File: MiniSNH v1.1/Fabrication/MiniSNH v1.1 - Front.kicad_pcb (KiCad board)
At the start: 2 copper layers, 20 x 128.5 mm, 11 parts

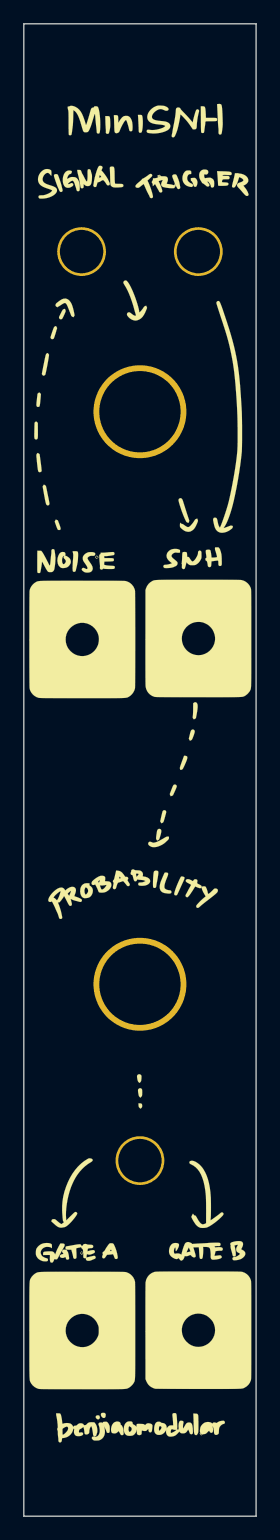
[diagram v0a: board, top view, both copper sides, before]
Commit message: Added gerber files for v1.1
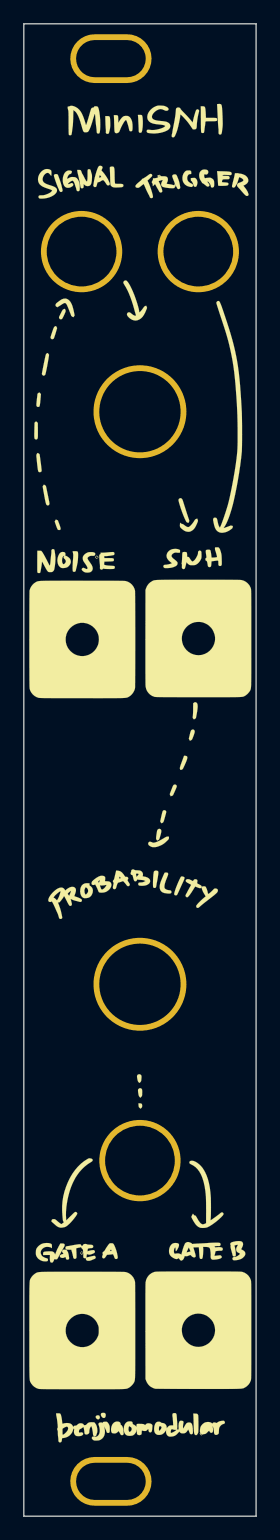
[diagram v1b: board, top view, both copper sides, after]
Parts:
- added REF**: Panel_4HP, benjiaomodular:Panel_4HP, F.Cu at (110.0, 49.0)
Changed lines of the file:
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@@
   )
   (paper "A4")
+  (title_block
+    (title "MiniSNH")
+    (date "2023-06-07")
+    (rev "V1.1")
+    (company "benjiaomodular")
+  )
   (layers
     (0 "F.Cu" signal)
@@
     )
     (pad_to_mask_clearance 0)
-    (grid_origin 110 49)
     (pcbplotparams
       (layerselection 0x00010fc_ffffffff)
@@
       (drillshape 0)
       (scaleselection 1)
-      (outputdirectory "")
+      (outputdirectory "./MiniSNH v1.1 - Front")
     )
   )
@@
       (effects (font (size 1.27 1.27) (thickness 0.15)))
     )
-    (pad "1" thru_hole circle locked (at 0 0) (size 4.2 4.2) (drill 3.735001) (layers *.Cu *.Mask))
+    (pad "1" thru_hole circle locked (at 0 0) (size 7 7) (drill 6) (layers *.Cu *.Mask))
   )
   (footprint "Wire_Pads:SolderWirePad_single_0-8mmDrill" (layer "F.Cu")
@@
       (effects (font (size 1.27 1.27) (thickness 0.15)))
     )
-    (pad "5" thru_hole circle locked (at 0 0) (size 4.2 4.2) (drill 3.735001) (layers *.Cu *.Mask))
+    (pad "5" thru_hole circle locked (at 0 0) (size 7 7) (drill 6) (layers *.Cu *.Mask))
   )
   (footprint "LOGO" (layer "F.Cu")
@@
       (effects (font (size 1.27 1.27) (thickness 0.15)))
     )
-    (pad "3" thru_hole circle locked (at 0 0) (size 4.2 4.2) (drill 3.735001) (layers *.Cu *.Mask))
+    (pad "3" thru_hole circle locked (at 0 0) (size 7 7) (drill 6) (layers *.Cu *.Mask))
   )
   (footprint "LOGO" (layer "F.Cu")
@@
       ) (layer "F.Mask") (width 0.01) (fill solid))
   )
+  (footprint "benjiaomodular:Panel_4HP" (layer "F.Cu")
+    (at 110 49)
+    (attr through_hole)
+    (fp_text reference "REF**" (at 18 -1) (layer "F.Fab") hide
+      (effects (font (size 1 1) (thickness 0.15)))
+    )
+    (fp_text value "Panel_4HP" (at 4 -1) (layer "F.Fab")
+      (effects (font (size 1 1) (thickness 0.15)))
+    )
+    (fp_text user "Clearance for 2020 Aluminum Extrusion" (at 10.5 11.5) (layer "Dwgs.User")
+      (effects (font (size 0.8 0.8) (thickness 0.12)))
+    )
+    (fp_text user "Clearance for 2020 Aluminum Extrusion" (at 10.5 116.5) (layer "Dwgs.User")
+      (effects (font (size 0.8 0.8) (thickness 0.12)))
+    )
+    (fp_line (start 0 128.5) (end 0 0) (layer "Dwgs.User") (width 0.12))
+    (fp_line (start 20 0) (end 20 128.5) (layer "Dwgs.User") (width 0.12))
+    (fp_line (start 0 125.5) (end 20 125.5) (layer "Dwgs.User") (width 0.12))
+    (fp_line (start 0 13) (end 20 13) (layer "Dwgs.User") (width 0.12))
+    (fp_line (start 0 3) (end 20 3) (layer "Dwgs.User") (width 0.12))
+    (fp_line (start 0 115.5) (end 20 115.5) (layer "Dwgs.User") (width 0.12))
+    (fp_line (start 0 0) (end 20 0) (layer "Dwgs.User") (width 0.12))
+    (fp_line (start 20 128.5) (end 0 128.5) (layer "Dwgs.User") (width 0.12))
+    (pad "" thru_hole oval locked (at 7.5 125.5) (size 7 4.2) (drill oval 6 3.2) (layers *.Cu *.Mask))
+    (pad "" thru_hole oval locked (at 7.5 3) (size 7 4.2) (drill oval 6 3.2) (layers *.Cu *.Mask))
+  )
   (footprint "Wire_Pads:SolderWirePad_single_0-8mmDrill" (layer "F.Cu")
     (at 119.999999 146.882027)
@@
       (effects (font (size 1.27 1.27) (thickness 0.15)))
     )
-    (pad "4" thru_hole circle locked (at 0 0) (size 4.2 4.2) (drill 3.735001) (layers *.Cu *.Mask))
+    (pad "4" thru_hole circle locked (at 0 0) (size 7 7) (drill 6) (layers *.Cu *.Mask))
   )
   (footprint "Wire_Pads:SolderWirePad_single_0-8mmDrill" (layer "F.Cu")
@@
       (effects (font (size 1.27 1.27) (thickness 0.15)))
     )
-    (pad "2" thru_hole circle locked (at 0 0) (size 4.2 4.2) (drill 3.735001) (layers *.Cu *.Mask))
+    (pad "2" thru_hole circle locked (at 0 0) (size 7 7) (drill 6) (layers *.Cu *.Mask))
   )
   (footprint "Wire_Pads:SolderWirePad_single_0-8mmDrill" (layer "F.Cu")
@@
       (effects (font (size 1.27 1.27) (thickness 0.15)))
     )
-    (pad "6" thru_hole circle locked (at 0 0) (size 4.2 4.2) (drill 3.735001) (layers *.Cu *.Mask))
+    (pad "6" thru_hole circle locked (at 0 0) (size 7 7) (drill 6) (layers *.Cu *.Mask))
   )
   (footprint "Wire_Pads:SolderWirePad_single_0-8mmDrill" (layer "F.Cu")
@@
       (effects (font (size 1.27 1.27) (thickness 0.15)))
     )
-    (pad "7" thru_hole circle locked (at 0 0) (size 4.2 4.2) (drill 3.735001) (layers *.Cu *.Mask))
+    (pad "7" thru_hole circle locked (at 0 0) (size 7 7) (drill 6) (layers *.Cu *.Mask))
   )
   (footprint "Wire_Pads:SolderWirePad_single_0-8mmDrill" (layer "F.Cu")
